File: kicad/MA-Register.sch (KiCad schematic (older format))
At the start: 0 parts

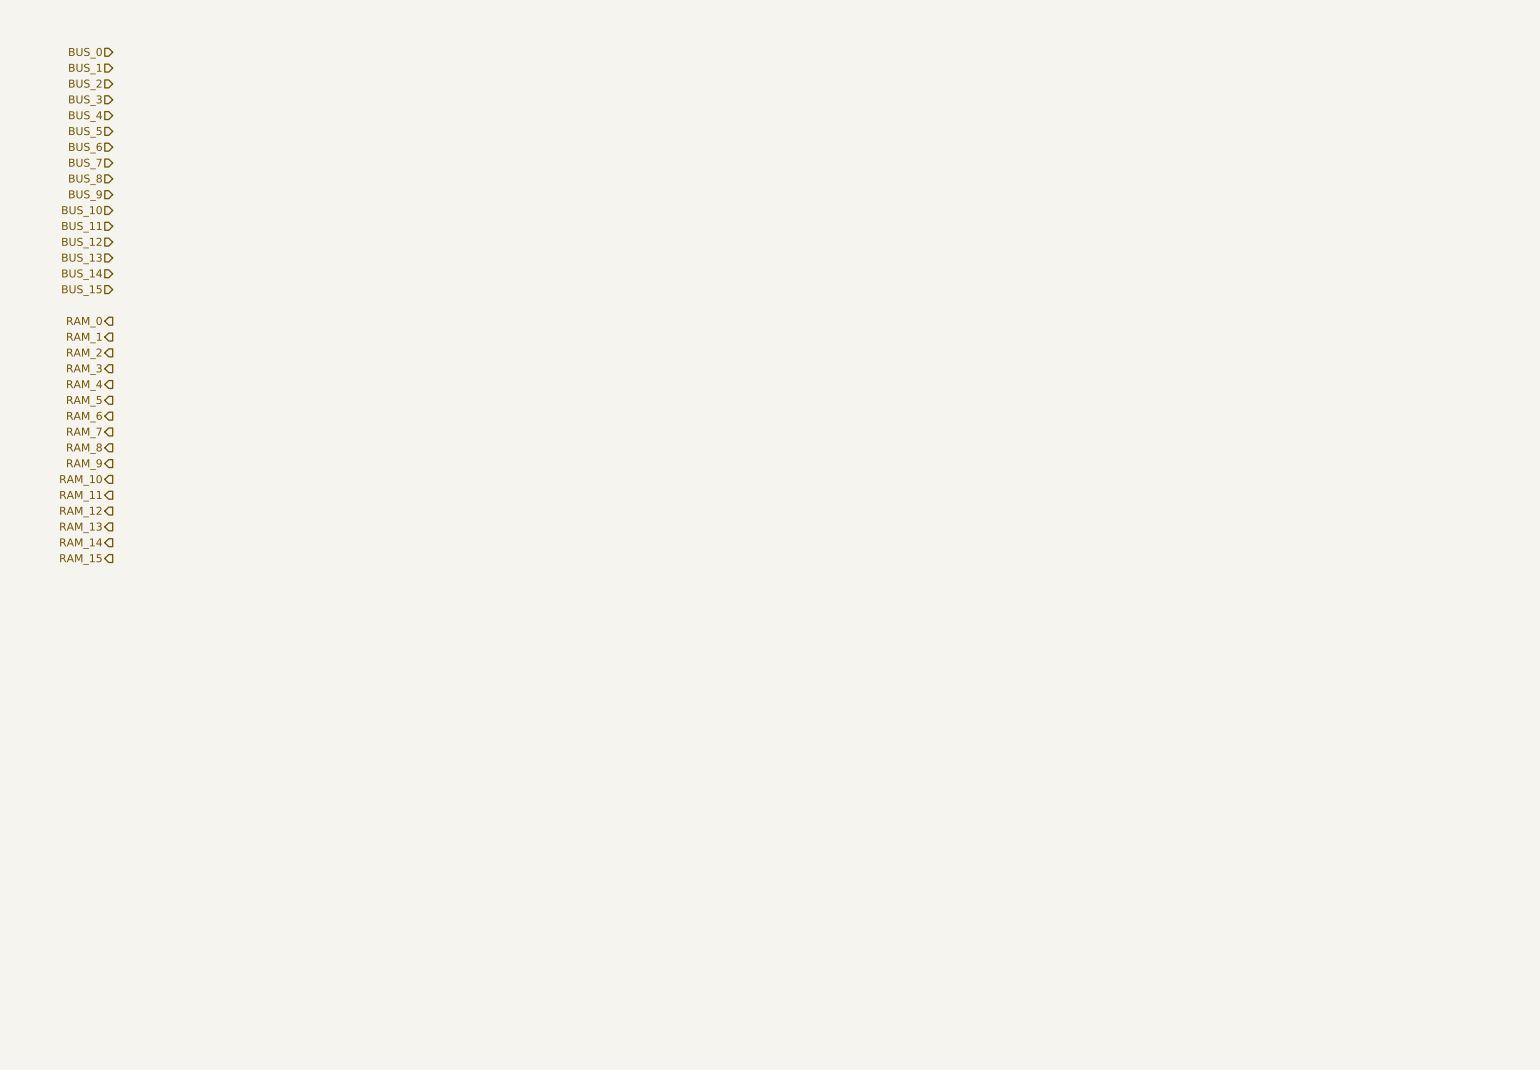
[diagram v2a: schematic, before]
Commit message: Finish todo list
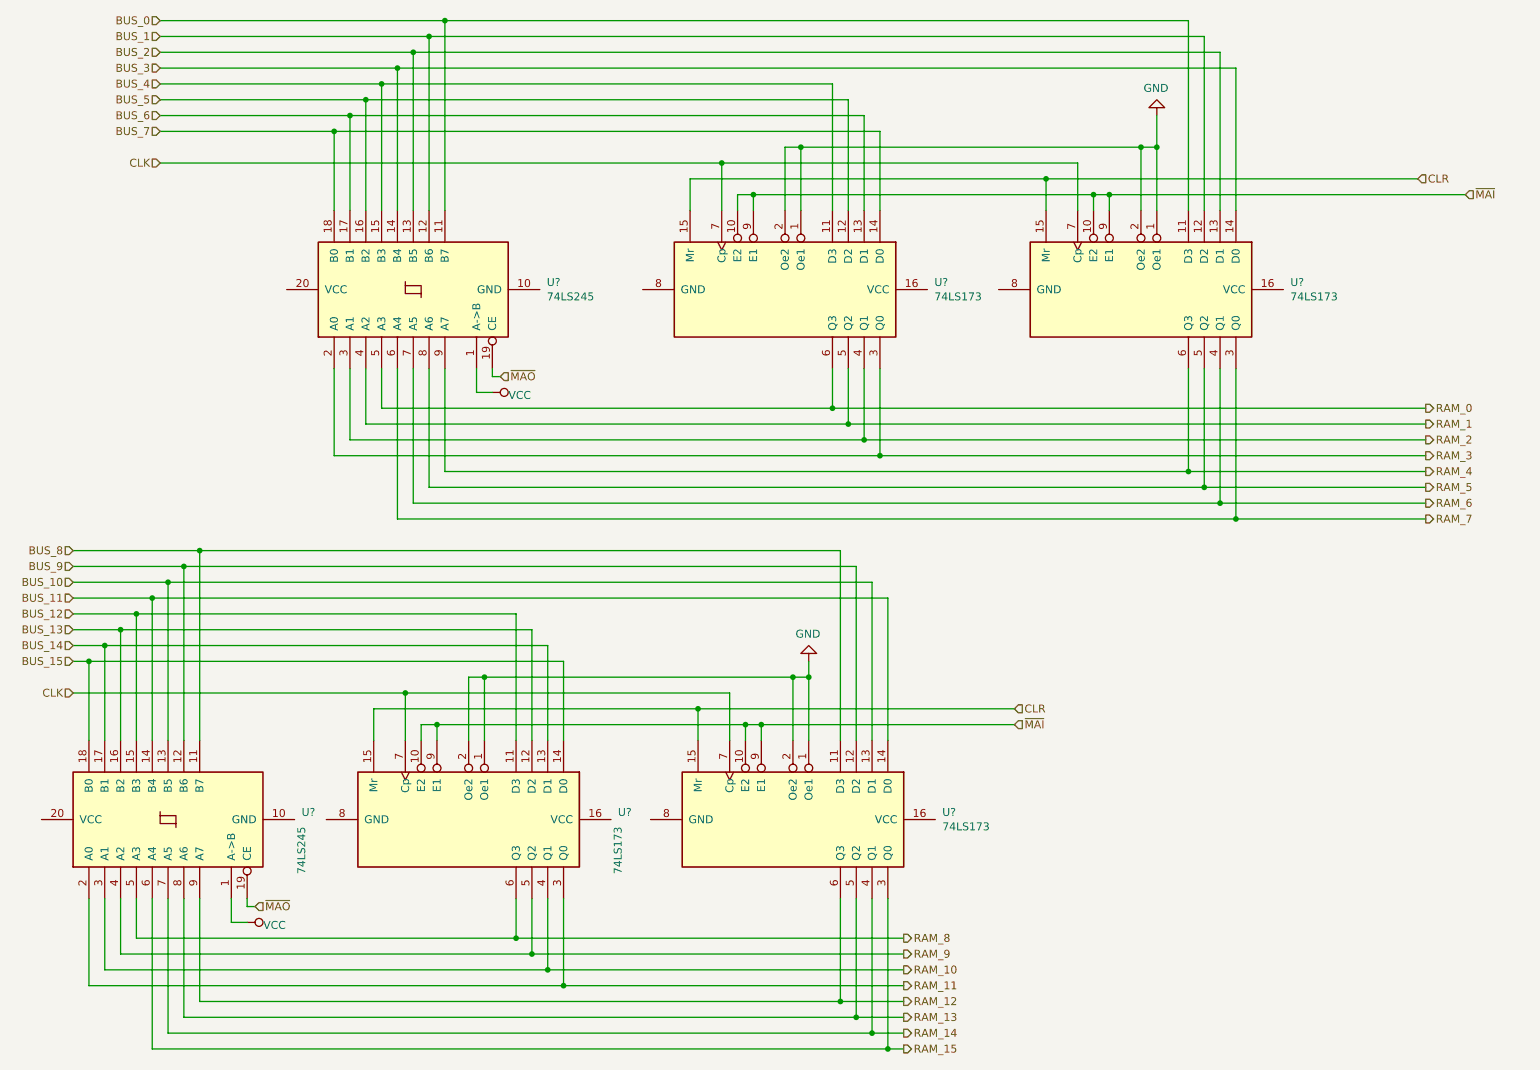
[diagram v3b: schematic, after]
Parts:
- added U? (x2): 74LS245, symbol 74xx:74LS245
- added U? (x4): 74LS173, symbol 74xx:74LS173
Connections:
- net BUS_0: now also U?.11 (B7), U?.11 (D3)
- net BUS_1: now also U?.12 (B6), U?.12 (D2)
- net BUS_10: now also U?.13 (B5), U?.13 (D1)
- net BUS_11: now also U?.14 (B4), U?.14 (D0)
- net BUS_12: now also U?.11 (D3), U?.15 (B3)
- net BUS_13: now also U?.12 (D2), U?.16 (B2)
- net BUS_14: now also U?.13 (D1), U?.17 (B1)
- net BUS_15: now also U?.14 (D0), U?.18 (B0)
- net BUS_2: now also U?.13 (B5), U?.13 (D1)
- net BUS_3: now also U?.14 (B4), U?.14 (D0)
- net BUS_4: now also U?.11 (D3), U?.15 (B3)
- net BUS_5: now also U?.12 (D2), U?.16 (B2)
- net BUS_6: now also U?.13 (D1), U?.17 (B1)
- net BUS_7: now also U?.14 (D0), U?.18 (B0)
- net BUS_8: now also U?.11 (B7), U?.11 (D3)
- net BUS_9: now also U?.12 (B6), U?.12 (D2)
- net RAM_0: now also U?.5 (A3), U?.6 (Q3)
- net RAM_1: now also U?.4 (A2), U?.5 (Q2)
- net RAM_10: now also U?.3 (A1), U?.4 (Q1)
- net RAM_11: now also U?.2 (A0), U?.3 (Q0)
- net RAM_12: now also U?.6 (Q3), U?.9 (A7)
- net RAM_13: now also U?.5 (Q2), U?.8 (A6)
- net RAM_14: now also U?.4 (Q1), U?.7 (A5)
- net RAM_15: now also U?.3 (Q0), U?.6 (A4)
- net RAM_2: now also U?.3 (A1), U?.4 (Q1)
- net RAM_3: now also U?.2 (A0), U?.3 (Q0)
- net RAM_4: now also U?.6 (Q3), U?.9 (A7)
- net RAM_5: now also U?.5 (Q2), U?.8 (A6)
- net RAM_6: now also U?.4 (Q1), U?.7 (A5)
- net RAM_7: now also U?.3 (Q0), U?.6 (A4)
- net RAM_8: now also U?.5 (A3), U?.6 (Q3)
- net RAM_9: now also U?.4 (A2), U?.5 (Q2)
- new net CLK: U?.7 (Cp), U?.7 (Cp), U?.7 (Cp), U?.7 (Cp)
- new net CLR: U?.15 (Mr), U?.15 (Mr), U?.15 (Mr), U?.15 (Mr)
- new net GND: U?.1 (Oe1), U?.1 (Oe1), U?.1 (Oe1), U?.1 (Oe1), U?.2 (Oe2), U?.2 (Oe2), U?.2 (Oe2), U?.2 (Oe2)
- new net VCC: U?.1 (A->B), U?.1 (A->B)
- new net ~MAI~: U?.10 (E2), U?.10 (E2), U?.10 (E2), U?.10 (E2), U?.9 (E1), U?.9 (E1), U?.9 (E1), U?.9 (E1)
- new net ~MAO~: U?.19 (CE), U?.19 (CE)
